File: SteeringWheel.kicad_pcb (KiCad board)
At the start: 2 copper layers, 22 parts

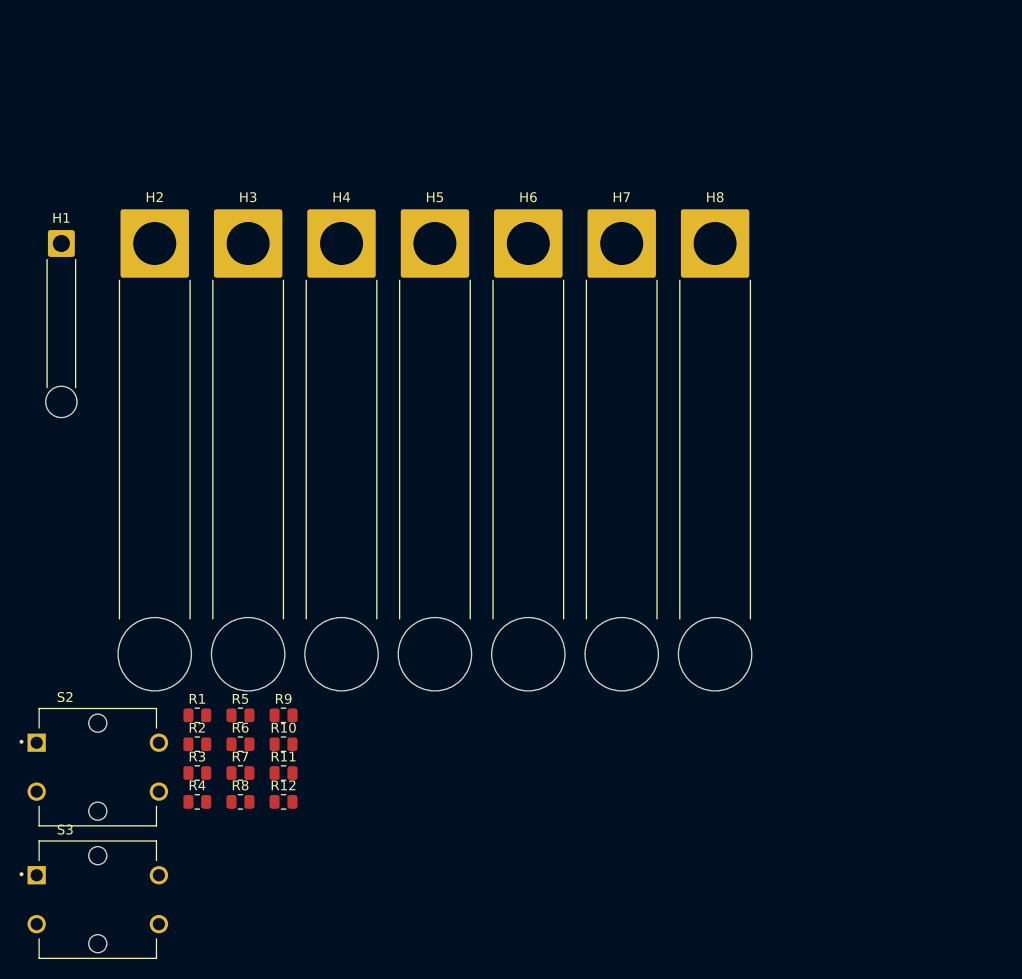
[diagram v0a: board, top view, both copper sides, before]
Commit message: Component Placement Finished
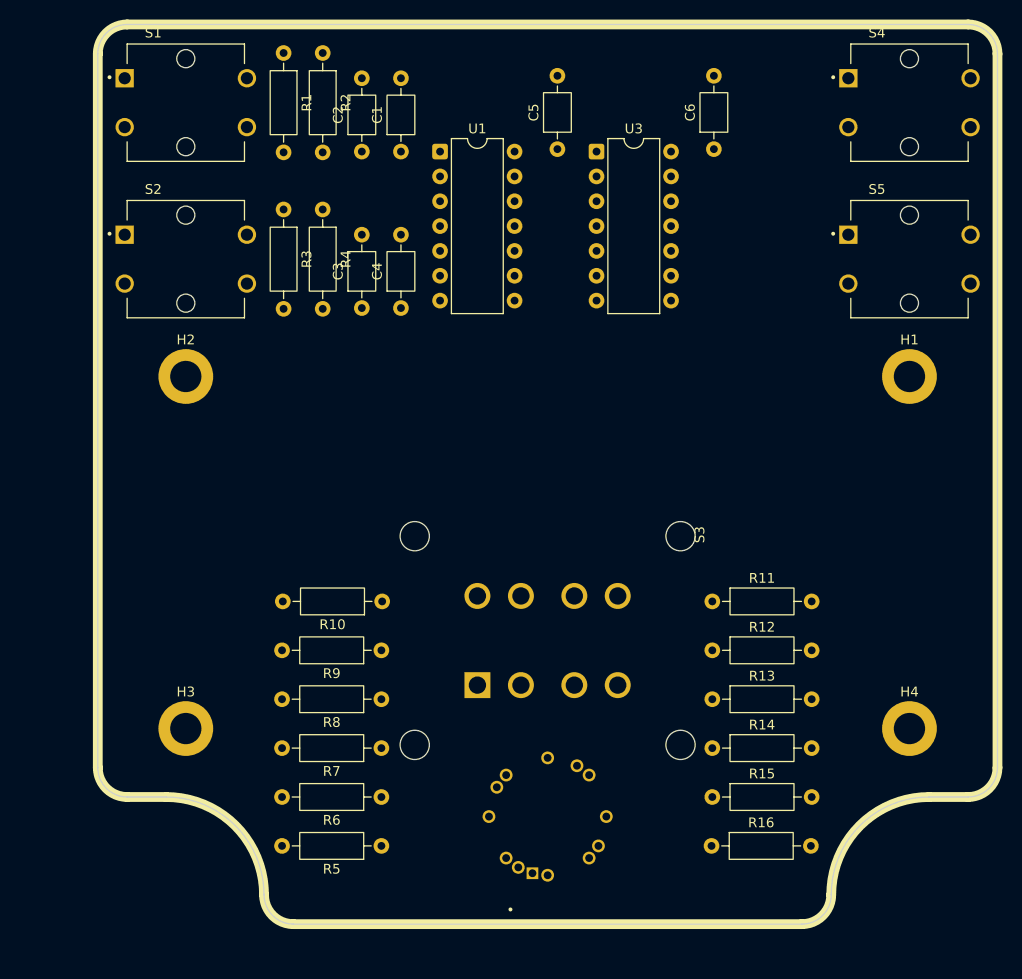
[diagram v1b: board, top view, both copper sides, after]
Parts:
- removed H5, H6, H7, H8: MountingHole_Pad, Connector_Wire:SolderWire-6sqmm_1x01_D3.5mm_OD7mm_Relief
- added C1: 100nF, Capacitor_THT:C_Axial_L3.8mm_D2.6mm_P7.50mm_Horizontal, F.Cu at (126.0, 52.0)
- added C2: 100nF, Capacitor_THT:C_Axial_L3.8mm_D2.6mm_P7.50mm_Horizontal, F.Cu at (122.0, 52.0)
- added C3: 100nF, Capacitor_THT:C_Axial_L3.8mm_D2.6mm_P7.50mm_Horizontal, F.Cu at (122.0, 68.0)
- added C4: 100nF, Capacitor_THT:C_Axial_L3.8mm_D2.6mm_P7.50mm_Horizontal, F.Cu at (126.0, 68.0)
- added C5: 100nF, Capacitor_THT:C_Axial_L3.8mm_D2.6mm_P7.50mm_Horizontal, F.Cu at (142.0, 51.8)
- added C6: 100nF, Capacitor_THT:C_Axial_L3.8mm_D2.6mm_P7.50mm_Horizontal, F.Cu at (158.0, 51.8)
- added J1: DT15-08PA, Connector_DTM:TE_DT15-08PA, B.Cu at (141.0, 102.0)
- added R13: 2430, Resistor_THT:R_Axial_DIN0207_L6.3mm_D2.5mm_P10.16mm_Horizontal, F.Cu at (157.8, 108.0)
- added R14: 3830, Resistor_THT:R_Axial_DIN0207_L6.3mm_D2.5mm_P10.16mm_Horizontal, F.Cu at (157.8, 113.0)
- added R15: 6980, Resistor_THT:R_Axial_DIN0207_L6.3mm_D2.5mm_P10.16mm_Horizontal, F.Cu at (157.8, 118.0)
- added R16: 23200, Resistor_THT:R_Axial_DIN0207_L6.3mm_D2.5mm_P10.16mm_Horizontal, F.Cu at (157.8, 123.0)
- added S1: B3F-4055, Button_Switch_THT:SW_B3F-4055, F.Cu at (104.0, 47.0)
- added S4: B3F-4055, Button_Switch_THT:SW_B3F-4055, F.Cu at (178.0, 47.0)
- added S5: B3F-4055, Button_Switch_THT:SW_B3F-4055, F.Cu at (178.0, 63.0)
- added U1: 74HC7014, Package_DIP:DIP-14_W7.62mm, F.Cu at (130.0, 52.0)
- added U3: 74HCT74, Package_DIP:DIP-14_W7.62mm, F.Cu at (146.0, 52.0)
- H1: value MountingHole_Pad -> MountingHole_Pad_MP; footprint Connector_Wire:SolderWire-1sqmm_1x01_D1.4mm_OD2.7mm_Relief -> MountingHole:MountingHole_3.2mm_M3_DIN965_Pad
- H2, H3, H4: value MountingHole_Pad -> MountingHole_Pad_MP; footprint Connector_Wire:SolderWire-6sqmm_1x01_D3.5mm_OD7mm_Relief -> MountingHole:MountingHole_3.2mm_M3_DIN965_Pad
- R1: value 43.2 -> 10k; footprint Resistor_SMD:R_0805_2012Metric -> Resistor_THT:R_Axial_DIN0207_L6.3mm_D2.5mm_P10.16mm_Horizontal
- R10: value 3830 -> 845; footprint Resistor_SMD:R_0805_2012Metric -> Resistor_THT:R_Axial_DIN0207_L6.3mm_D2.5mm_P10.16mm_Horizontal
- R11: value 6980 -> 1180; footprint Resistor_SMD:R_0805_2012Metric -> Resistor_THT:R_Axial_DIN0207_L6.3mm_D2.5mm_P10.16mm_Horizontal
- R12: value 23200 -> 1650; footprint Resistor_SMD:R_0805_2012Metric -> Resistor_THT:R_Axial_DIN0207_L6.3mm_D2.5mm_P10.16mm_Horizontal
- R2: value 143 -> 100k; footprint Resistor_SMD:R_0805_2012Metric -> Resistor_THT:R_Axial_DIN0207_L6.3mm_D2.5mm_P10.16mm_Horizontal
- R3: value 261 -> 10k; footprint Resistor_SMD:R_0805_2012Metric -> Resistor_THT:R_Axial_DIN0207_L6.3mm_D2.5mm_P10.16mm_Horizontal
- R4: value 412 -> 100k; footprint Resistor_SMD:R_0805_2012Metric -> Resistor_THT:R_Axial_DIN0207_L6.3mm_D2.5mm_P10.16mm_Horizontal
- R5: value 604 -> 43.2; footprint Resistor_SMD:R_0805_2012Metric -> Resistor_THT:R_Axial_DIN0207_L6.3mm_D2.5mm_P10.16mm_Horizontal
- R6: value 845 -> 143; footprint Resistor_SMD:R_0805_2012Metric -> Resistor_THT:R_Axial_DIN0207_L6.3mm_D2.5mm_P10.16mm_Horizontal
- R7: value 1180 -> 261; footprint Resistor_SMD:R_0805_2012Metric -> Resistor_THT:R_Axial_DIN0207_L6.3mm_D2.5mm_P10.16mm_Horizontal
- R8: value 1650 -> 412; footprint Resistor_SMD:R_0805_2012Metric -> Resistor_THT:R_Axial_DIN0207_L6.3mm_D2.5mm_P10.16mm_Horizontal
- R9: value 2430 -> 604; footprint Resistor_SMD:R_0805_2012Metric -> Resistor_THT:R_Axial_DIN0207_L6.3mm_D2.5mm_P10.16mm_Horizontal
- S3: value B3F-4055 -> MRK112-A; footprint Button_Switch_THT:SW_B3F-4055 -> MRK112_A (3):SW_MRK112-A
- moved H1 87.8 mm to (178.0, 75.0)
- moved H4 76.4 mm to (178.0, 111.0)
- moved R2 71.8 mm to (118.0, 41.9), turned to -90 degrees
- moved R1 68.3 mm to (114.0, 41.9), turned to -90 degrees
- moved R4 61.9 mm to (118.0, 57.9), turned to -90 degrees
- moved R3 58.3 mm to (114.0, 57.9), turned to -90 degrees
- moved S2 52.7 mm to (104.0, 63.0)
- moved H3 50.0 mm to (104.0, 111.0)
- moved R11 47.2 mm to (157.8, 98.0)
- moved S3 46.8 mm to (141.0, 120.0)
- moved R12 46.5 mm to (157.8, 103.0)
- moved R5 19.6 mm to (124.0, 123.0), turned to 180 degrees
- moved R8 17.8 mm to (124.0, 108.0), turned to 180 degrees
- moved R10 17.7 mm to (124.1, 98.0), turned to 180 degrees
- moved R6 15.4 mm to (124.0, 118.0), turned to 180 degrees
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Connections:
- H1 pad 1: unconnected-(H1-Pad1) -> (no net)
- H2 pad 1: unconnected-(H2-Pad1) -> (no net)
- H3 pad 1: unconnected-(H3-Pad1) -> (no net)
- H4 pad 1: unconnected-(H4-Pad1) -> (no net)
- R1 pad 1: Net-(R1-Pad1) -> +5V
- R1 pad 2: GND -> Net-(C1-Pad1)
- R2 pad 1: Net-(R2-Pad1) -> +5V
- R2 pad 2: GND -> Net-(C2-Pad1)
- R3 pad 1: Net-(R3-Pad1) -> +5V
- R3 pad 2: GND -> Net-(C3-Pad1)
- R4 pad 1: Net-(R4-Pad1) -> +5V
- R4 pad 2: GND -> Net-(C4-Pad1)
- S2 pad 1: Net-(S2-Pad1) -> GND
- S2 pad 2: Net-(S2-Pad1) -> GND
- S2 pad 3: /MCU/Fuel Reset -> Net-(C3-Pad1)
- S2 pad 4: /MCU/Fuel Reset -> Net-(C3-Pad1)
- S3 pad 1: Net-(S3-Pad1) -> Net-(R5-Pad1)
- S3 pad 2: Net-(S3-Pad1) -> Net-(R6-Pad1)
- S3 pad 3: Net-(S3-Pad3) -> Net-(R7-Pad1)
- S3 pad 4: Net-(S3-Pad3) -> Net-(R8-Pad1)
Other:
- board outline added: 92 x 92 mm
- board text added: "For Instructional Use Only."
- board text added: "SOLIDWORKS Educational Product."
